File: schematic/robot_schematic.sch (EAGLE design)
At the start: 4 parts

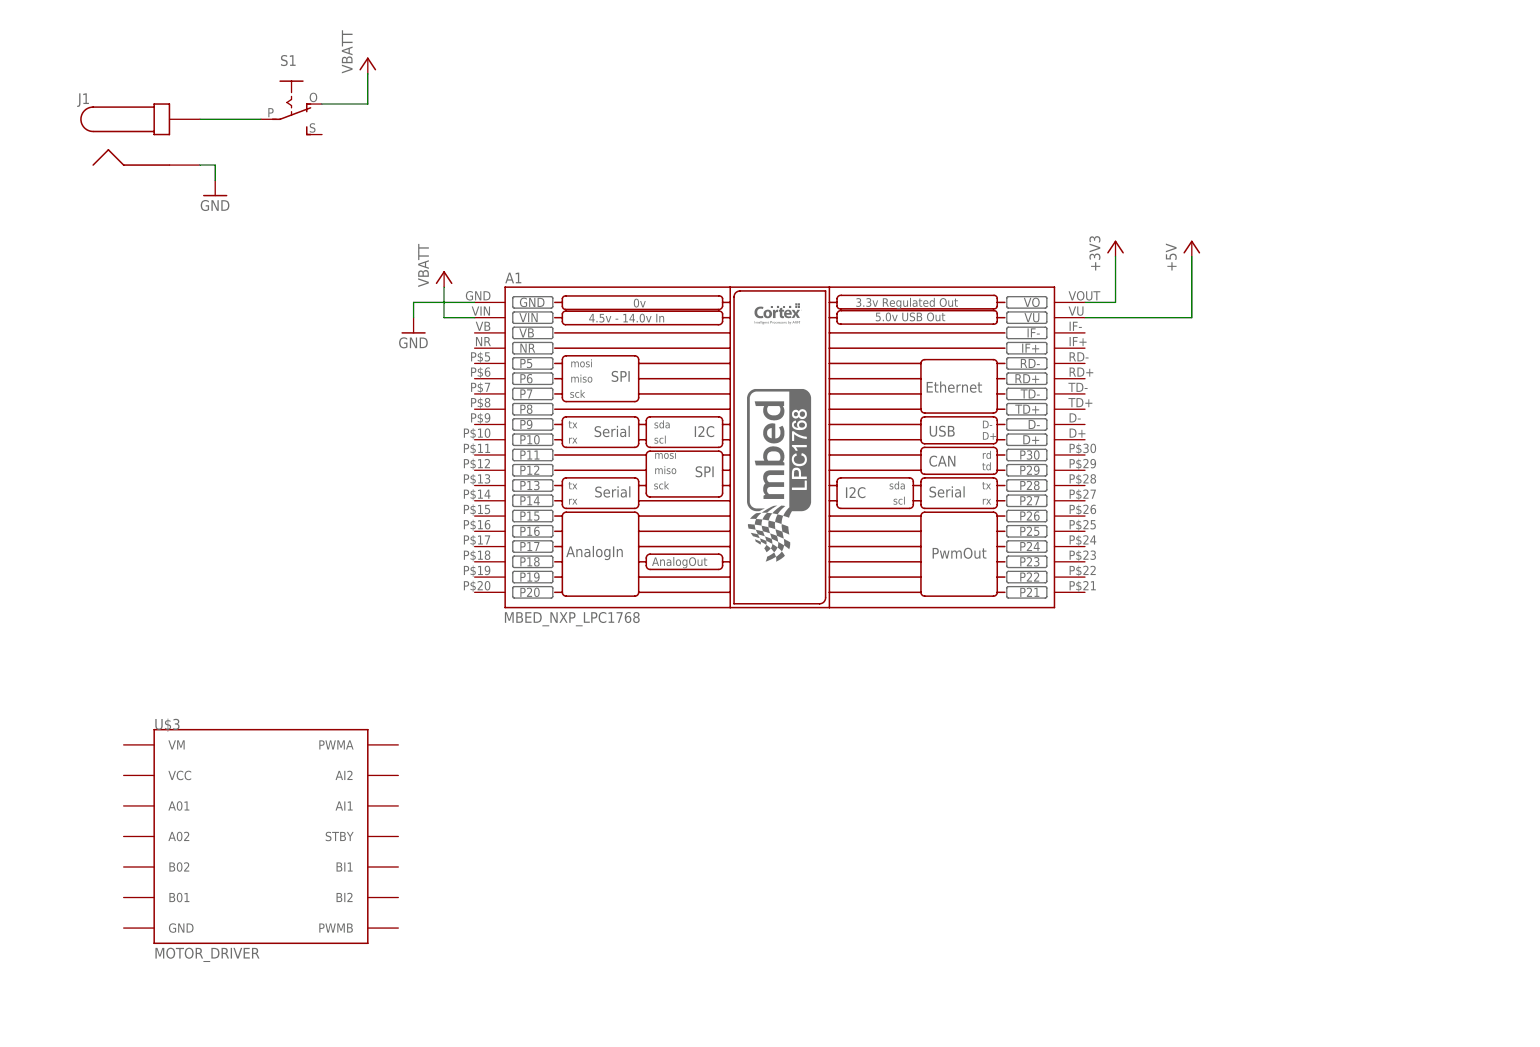
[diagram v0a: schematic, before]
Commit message: finished schematic
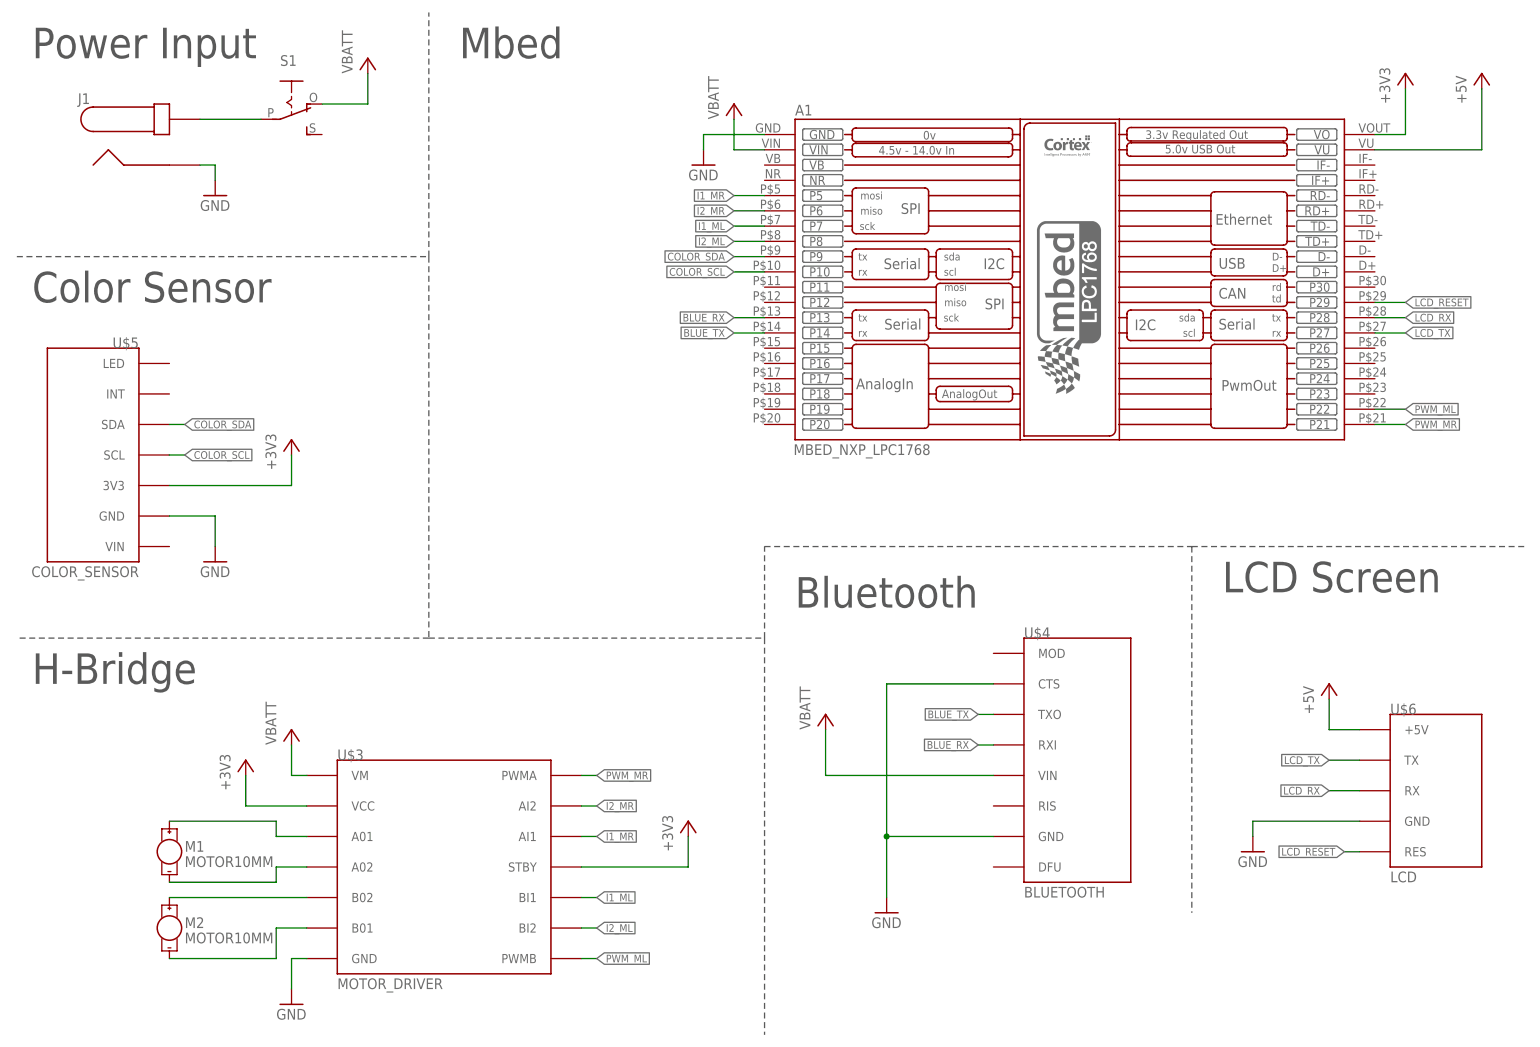
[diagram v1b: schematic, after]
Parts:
- added M1, M2: MOTOR10MM, SparkFun-Electromechanical:MOTOR10MM
- added U$4: BLUETOOTH, schematic_sym:BLUETOOTH
- added U$5: COLOR_SENSOR, schematic_sym:COLOR_SENSOR
- added U$6: LCD, schematic_sym:LCD
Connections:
- new net BLUE_RX: A1.P13, U$4.RXI
- new net BLUE_TX: A1.P14, U$4.TXO
- new net COLOR_SCL: A1.P10, U$5.SCL
- new net COLOR_SDA: A1.P9, U$5.SDA
- new net I1_ML: A1.P7, U$3.BI1
- new net I1_MR: A1.P5, U$3.AI1
- new net I2_ML: A1.P8, U$3.BI2
- new net I2_MR: A1.P6, U$3.AI2
- new net LCD_RESET: A1.P29, U$6.RES
- new net LCD_RX: A1.P28, U$6.RX
- new net LCD_TX: A1.P27, U$6.TX
- new net N$2: M1.+, U$3.A01
- new net N$3: M1.-, U$3.A02
- new net N$4: M2.+, U$3.B02
- new net N$5: M2.-, U$3.B01
- new net PWM_ML: A1.P22, U$3.PWMB
- new net PWM_MR: A1.P21, U$3.PWMA
- net +3V3: now also U$3.STBY, U$3.VCC, U$5.3V3
- net +5V: now also U$6.+5V
- net GND: now also U$3.GND, U$4.CTS, U$4.GND, U$5.GND, U$6.GND
- net VBATT: now also U$3.VM, U$4.VIN
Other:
- note added: "Bluetooth"
- note added: "Color Sensor"
- note added: "H-Bridge"
- note added: "LCD Screen"
- note added: "Mbed"
- note added: "Power Input"
- moved on the sheet: A1, U$3
